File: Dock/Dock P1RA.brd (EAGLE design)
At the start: 51 x 40 mm, 14 parts, among them J2 MF-CON-2.54mm-01x07, J3 MF-CON-2.54mm-01x05, U1 MCP73831T-2ACI/OT

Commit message: increased holes to 3mm
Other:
- board text added: "http://tilestoolkit.io Prototype 1 Rev. A simone.mora@ntnu.no"
- board text removed: "http://tilestoolkit.io Prototype 1 Rev. A Simone Mora (simonem@ntnu.no)"
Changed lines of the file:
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@@
 <text x="18.8722" y="-36.957" size="1" layer="22" font="vector" rot="MR0" align="center">http://tilestoolkit.io
 Prototype 1 Rev. A
-Simone Mora (simonem@ntnu.no)</text>
+simone.mora@ntnu.no</text>
 <rectangle x1="12.98" y1="-30.02" x2="13.26" y2="-29.98" layer="22"/>
 <rectangle x1="12.9" y1="-29.98" x2="13.34" y2="-29.94" layer="22"/>

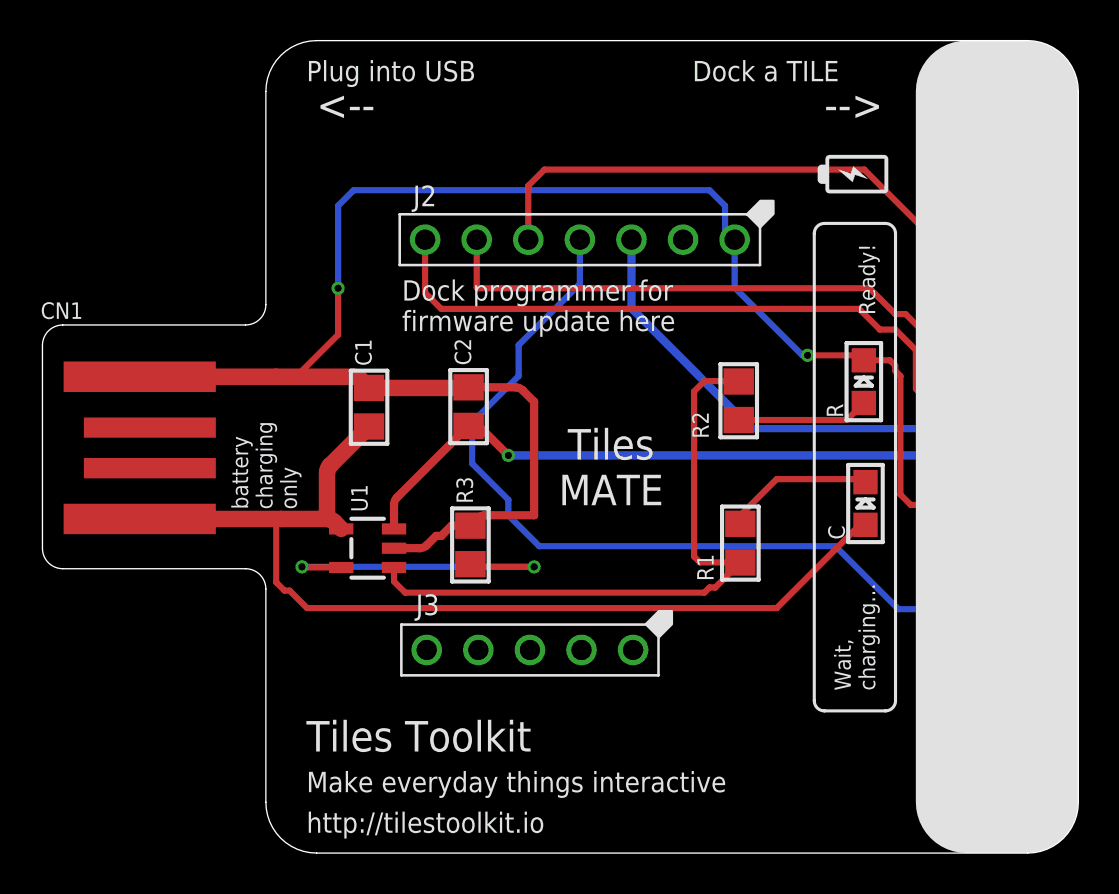
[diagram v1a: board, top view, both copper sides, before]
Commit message: candidate p3 and dock
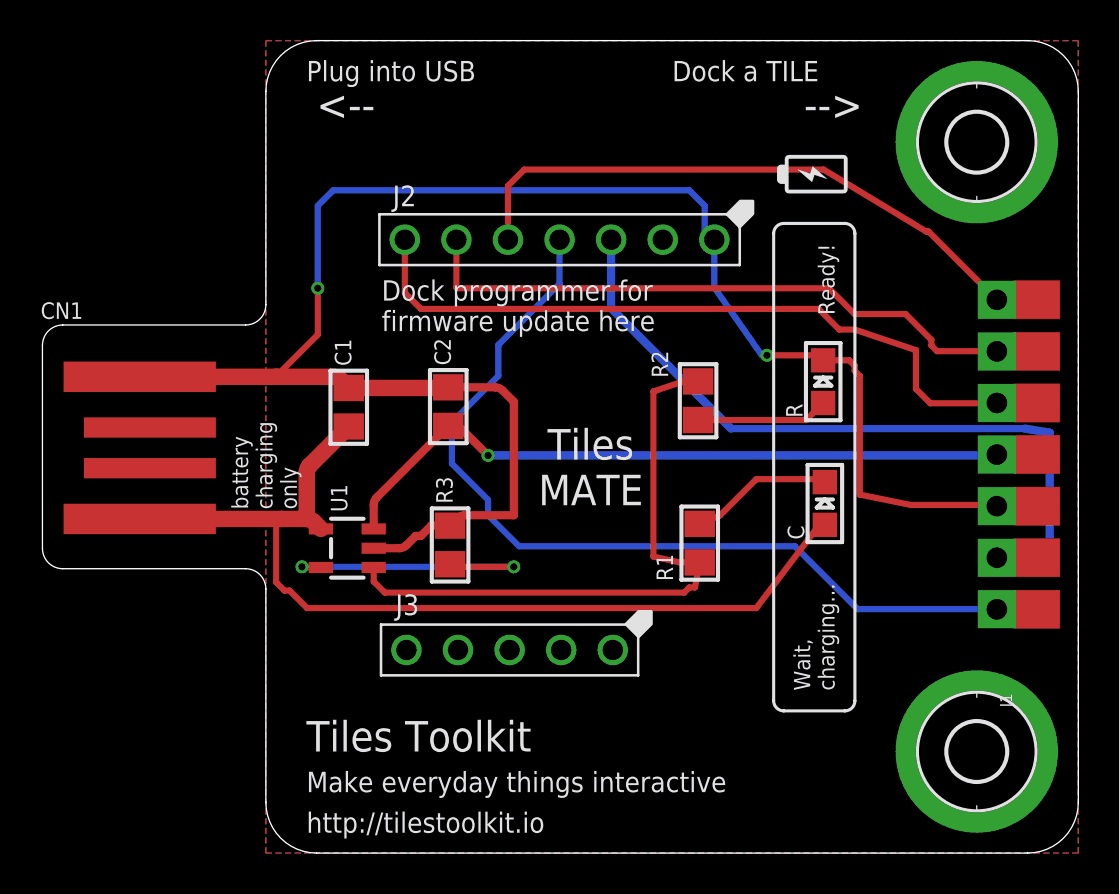
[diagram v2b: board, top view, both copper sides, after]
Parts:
- moved C 2.00 mm to (27.5, -22.8)
- moved R 2.00 mm to (27.4, -16.8)
- moved R1 2.00 mm to (21.4, -24.7)
- moved R2 2.00 mm to (21.3, -17.7)
- moved H1 1.41 mm to (35.0, -5.00)
- moved H2 1.41 mm to (35.0, -35.0)
- moved C1 1.00 mm to (4.08, -18.1)
- moved C2 1.00 mm to (8.98, -18.0)
- moved J2 1.00 mm to (14.5, -9.80)
- moved J3 1.00 mm to (12.0, -30.0)
- moved R3 1.00 mm to (9.07, -24.8)
- moved U1 1.00 mm to (4.01, -25.0)
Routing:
- net VCC: track 32.9 -> 35.9 mm
- net VDD: track 49.9 -> 47.3 mm
- net N$5: track 16.6 -> 14.6 mm
- net VBAT: track 33.2 -> 34.2 mm
- net RESET: track 42.5 -> 43.5 mm
- net GPIO0(TX): track 29.4 -> 30.4 mm
- net GND: track 88.1 -> 87.3 mm
- net GPIO1(RX): track 34.1 -> 34.9 mm
- net N$2: track 31.5 -> 30.8 mm
- net FACTORY: track 28.7 -> 29.3 mm
- added copper zone on layer 1, net GND
- added copper zone on layer 16, net GND
